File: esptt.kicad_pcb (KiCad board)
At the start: 2 copper layers, 21.3 x 43 mm, 17 parts

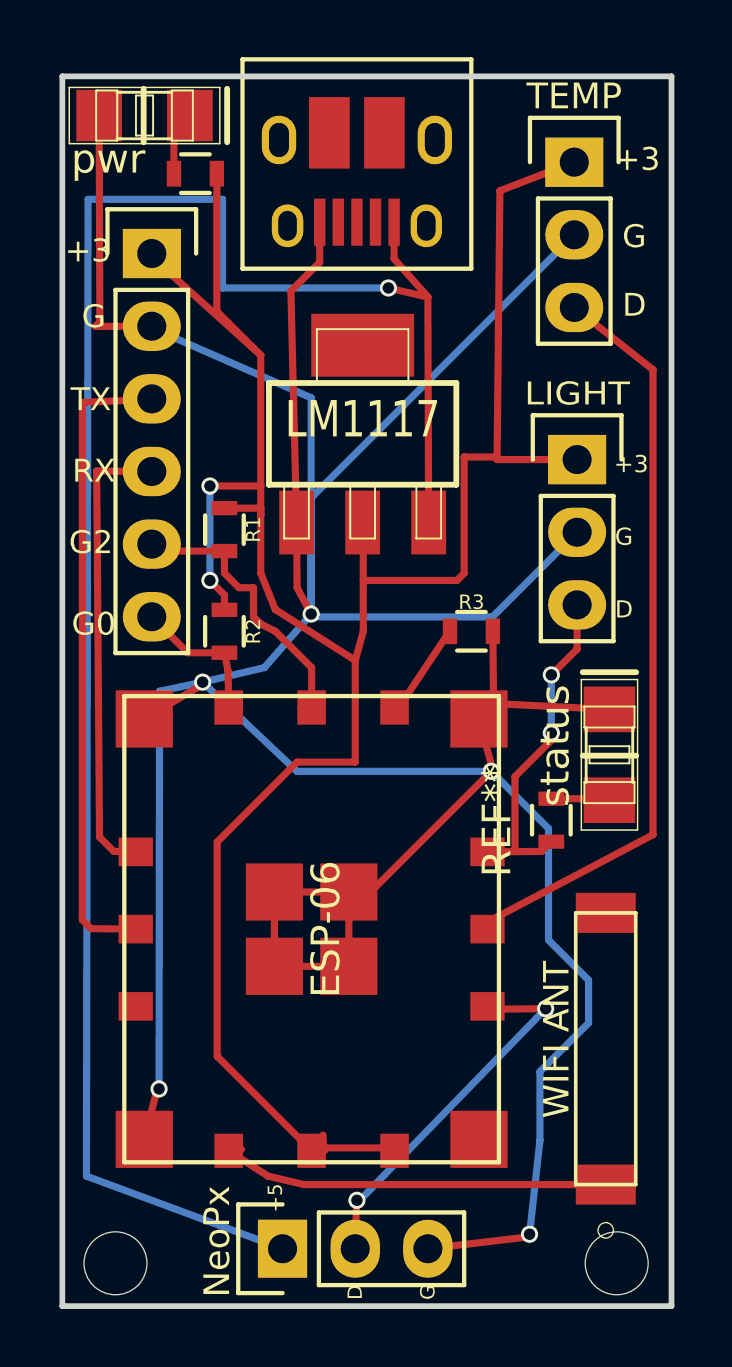
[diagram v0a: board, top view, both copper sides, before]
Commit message: updated eps-06 part
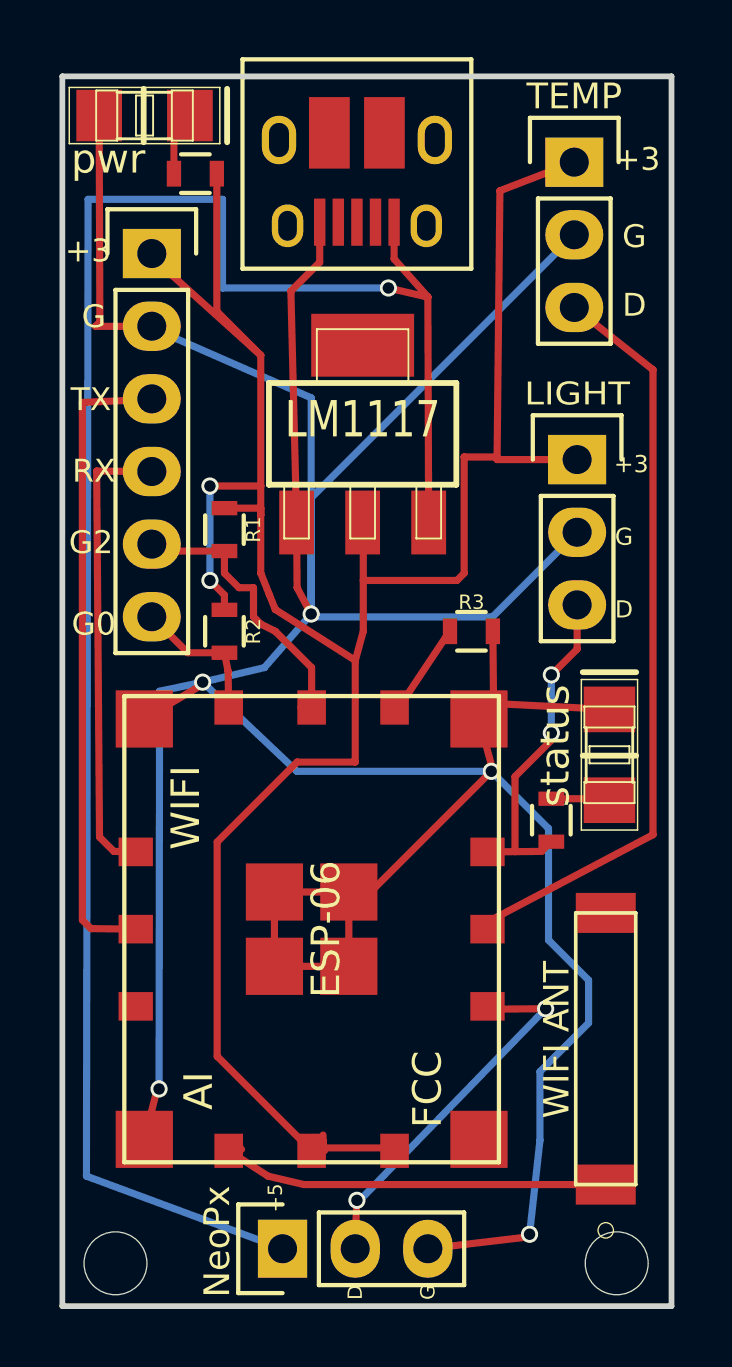
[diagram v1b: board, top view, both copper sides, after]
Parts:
- ESP-06: footprint ESP-06 -> ESP8266:ESP-06
- renumbered REF** to ?
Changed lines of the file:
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@@
     (32 B.Adhes user)
     (33 F.Adhes user)
-    (34 B.Paste user hide)
+    (34 B.Paste user)
     (35 F.Paste user)
     (36 B.SilkS user hide)
@@
     (pad 2 smd rect (at 4.7498 0 90) (size 1.39954 2.09804) (layers F.Cu F.Paste F.Mask))
   )
-  (module ESP-06 (layer F.Cu)
-    (at 140.716 67.818 90)
-    (fp_text reference ESP-06 (at 0 0.5 90) (layer F.SilkS)
-      (effects (font (size 1 1) (thickness 0.15)))
-    )
-    (fp_text value ESP-06 (at 0 -0.5 90) (layer F.Fab) hide
-      (effects (font (size 1 1) (thickness 0.15)))
-    )
-    (fp_line (start -8.15 6.55) (end 8.15 6.55) (layer F.SilkS) (width 0.15))
-    (fp_line (start 8.15 6.55) (end 8.15 -6.55) (layer F.SilkS) (width 0.15))
-    (fp_line (start 8.15 -6.55) (end -8.15 -6.55) (layer F.SilkS) (width 0.15))
-    (fp_line (start -8.15 -6.55) (end -8.15 6.55) (layer F.SilkS) (width 0.15))
-    (pad G smd rect (at -7.35 -5.85 90) (size 2 2) (layers F.Cu F.Paste F.Mask))
-    (pad G smd rect (at 7.35 -5.85 90) (size 2 2) (layers F.Cu F.Paste F.Mask))
-    (pad G smd rect (at -7.35 5.85 90) (size 2 2) (layers F.Cu F.Paste F.Mask))
-    (pad G smd rect (at 7.35 5.85 90) (size 2 2) (layers F.Cu F.Paste F.Mask))
-    (pad GP14 smd rect (at -2.7 6.15 90) (size 1 1.2) (layers F.Cu F.Paste F.Mask))
-    (pad GP13 smd rect (at 0 6.15 90) (size 1 1.2) (layers F.Cu F.Paste F.Mask))
-    (pad GP12 smd rect (at 2.7 6.15 90) (size 1 1.2) (layers F.Cu F.Paste F.Mask))
-    (pad TX smd rect (at 0 -6.15 90) (size 1 1.2) (layers F.Cu F.Paste F.Mask))
-    (pad GP16 smd rect (at -2.7 -6.15 90) (size 1 1.2) (layers F.Cu F.Paste F.Mask))
-    (pad RX smd rect (at 2.7 -6.15 90) (size 1 1.2) (layers F.Cu F.Paste F.Mask))
-    (pad 3.3 smd rect (at -7.75 0 90) (size 1.2 1) (layers F.Cu F.Paste F.Mask))
-    (pad CHPD smd rect (at -7.75 2.9 90) (size 1.2 1) (layers F.Cu F.Paste F.Mask))
-    (pad ANT smd rect (at -7.75 -2.9 90) (size 1.2 1) (layers F.Cu F.Paste F.Mask))
-    (pad GP2 smd rect (at 7.75 0 90) (size 1.2 1) (layers F.Cu F.Paste F.Mask))
-    (pad GP0 smd rect (at 7.75 -2.9 90) (size 1.2 1) (layers F.Cu F.Paste F.Mask))
-    (pad GP15 smd rect (at 7.75 2.9 90) (size 1.2 1) (layers F.Cu F.Paste F.Mask))
-    (pad Gx smd rect (at -1.3 -1.3 90) (size 2 2) (layers F.Cu F.Paste F.Mask))
-    (pad Gx smd rect (at 1.3 -1.3 90) (size 2 2) (layers F.Cu F.Paste F.Mask))
-    (pad Gx smd rect (at -1.3 1.3 90) (size 2 2) (layers F.Cu F.Paste F.Mask))
-    (pad Gx smd rect (at 1.3 1.3 90) (size 2 2) (layers F.Cu F.Paste F.Mask))
-  )
   (module Connect:USB_Micro-B_10103594-0001LF (layer F.Cu)
     (at 142.3 41.6 180)
@@
     (tags "resistor 0603")
     (attr smd)
-    (fp_text reference REF** (at 0 -1.9 90) (layer F.SilkS)
+    (fp_text reference "" (at 0 -1.9 90) (layer F.SilkS)
       (effects (font (size 1 1) (thickness 0.15)))
     )
@@
     (pad 1 np_thru_hole circle (at 0 0) (size 2.2 2.2) (drill 2.2) (layers *.Cu *.Mask F.SilkS))
   )
+  (module ESP8266:ESP-06 (layer F.Cu)
+    (at 140.716 67.818 90)
+    (fp_text reference ESP-06 (at 0 0.5 90) (layer F.SilkS)
+      (effects (font (size 1 1) (thickness 0.15)))
+    )
+    (fp_text value ESP-06 (at 0 -0.5 90) (layer F.Fab)
+      (effects (font (size 1 1) (thickness 0.15)))
+    )
+    (fp_text user AI (at -5.65 -3.95 90) (layer F.SilkS)
+      (effects (font (size 1 1) (thickness 0.15)))
+    )
+    (fp_text user WIFI (at 4.25 -4.4 90) (layer F.SilkS)
+      (effects (font (size 1 1) (thickness 0.15)))
+    )
+    (fp_text user FCC (at -5.6 4.05 90) (layer F.SilkS)
+      (effects (font (size 1 1) (thickness 0.15)))
+    )
+    (fp_line (start -8.15 6.55) (end 8.15 6.55) (layer F.SilkS) (width 0.15))
+    (fp_line (start 8.15 6.55) (end 8.15 -6.55) (layer F.SilkS) (width 0.15))
+    (fp_line (start 8.15 -6.55) (end -8.15 -6.55) (layer F.SilkS) (width 0.15))
+    (fp_line (start -8.15 -6.55) (end -8.15 6.55) (layer F.SilkS) (width 0.15))
+    (pad GND smd rect (at -7.35 -5.85 90) (size 2 2) (layers F.Cu F.Paste F.Mask))
+    (pad GP5 smd rect (at 7.35 -5.85 90) (size 2 2) (layers F.Cu F.Paste F.Mask))
+    (pad GP16 smd rect (at -7.35 5.85 90) (size 2 2) (layers F.Cu F.Paste F.Mask))
+    (pad GP15 smd rect (at 7.35 5.85 90) (size 2 2) (layers F.Cu F.Paste F.Mask))
+    (pad GP14 smd rect (at -2.7 6.15 90) (size 1 1.2) (layers F.Cu F.Paste F.Mask))
+    (pad GP12 smd rect (at 0 6.15 90) (size 1 1.2) (layers F.Cu F.Paste F.Mask))
+    (pad GP13 smd rect (at 2.7 6.15 90) (size 1 1.2) (layers F.Cu F.Paste F.Mask))
+    (pad TX smd rect (at 0 -6.15 90) (size 1 1.2) (layers F.Cu F.Paste F.Mask))
+    (pad RST smd rect (at -2.7 -6.15 90) (size 1 1.2) (layers F.Cu F.Paste F.Mask))
+    (pad RX smd rect (at 2.7 -6.15 90) (size 1 1.2) (layers F.Cu F.Paste F.Mask))
+    (pad 3.3 smd rect (at -7.75 0 90) (size 1.2 1) (layers F.Cu F.Paste F.Mask))
+    (pad CHPD smd rect (at -7.75 2.9 90) (size 1.2 1) (layers F.Cu F.Paste F.Mask))
+    (pad ANT smd rect (at -7.75 -2.9 90) (size 1.2 1) (layers F.Cu F.Paste F.Mask))
+    (pad GP2 smd rect (at 7.75 0 90) (size 1.2 1) (layers F.Cu F.Paste F.Mask))
+    (pad GP0 smd rect (at 7.75 -2.9 90) (size 1.2 1) (layers F.Cu F.Paste F.Mask))
+    (pad GP4 smd rect (at 7.75 2.9 90) (size 1.2 1) (layers F.Cu F.Paste F.Mask))
+    (pad GND smd rect (at -1.3 -1.3 90) (size 2 2) (layers F.Cu F.Paste F.Mask))
+    (pad GND smd rect (at 1.3 -1.3 90) (size 2 2) (layers F.Cu F.Paste F.Mask))
+    (pad GND smd rect (at -1.3 1.3 90) (size 2 2) (layers F.Cu F.Paste F.Mask))
+    (pad GND smd rect (at 1.3 1.3 90) (size 2 2) (layers F.Cu F.Paste F.Mask))
+  )
   (gr_text D (at 142.24 80.518 90) (layer F.SilkS)
